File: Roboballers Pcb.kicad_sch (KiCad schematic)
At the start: 79 parts, among them U1 TSOP25xx, U1 Teensy4.1, U10 TSOP25xx, U11 TSOP25xx, U12 TSOP25xx, U13 MCP3008, U14 TSOP25xx, U15 TSOP25xx, U16 TSOP25xx, U17 TSOP25xx, U18 TSOP25xx, U19 TSOP25xx, U2 TSOP25xx, U20 TSOP25xx, U21 TSOP25xx, U22 MCP3008, U23 TSOP25xx, U24 TSOP25xx, U25 TSOP25xx, U26 TSOP25xx, U3 TSOP25xx, U4 TSOP25xx, U5 TSOP25xx, U6 MCP3008, U6 TSOP25xx, U7 TSOP25xx, U8 TSOP25xx, U9 TSOP25xx

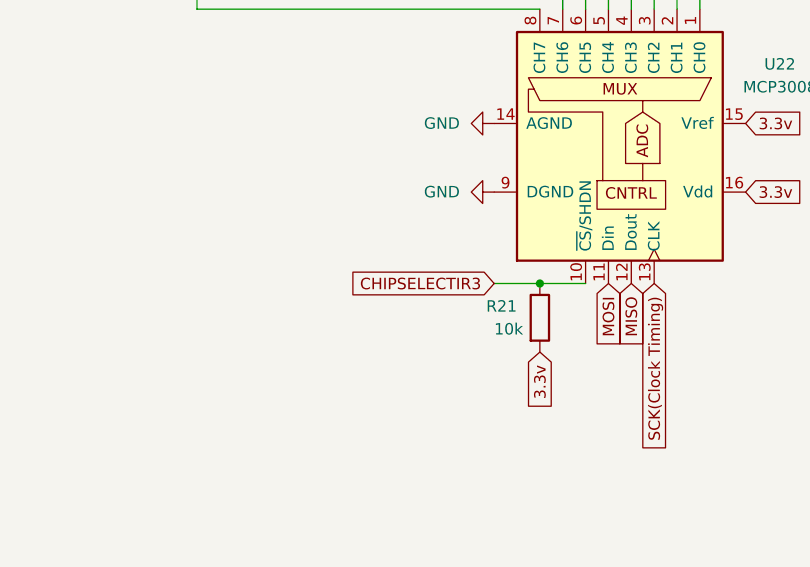
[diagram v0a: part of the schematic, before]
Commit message: Testing
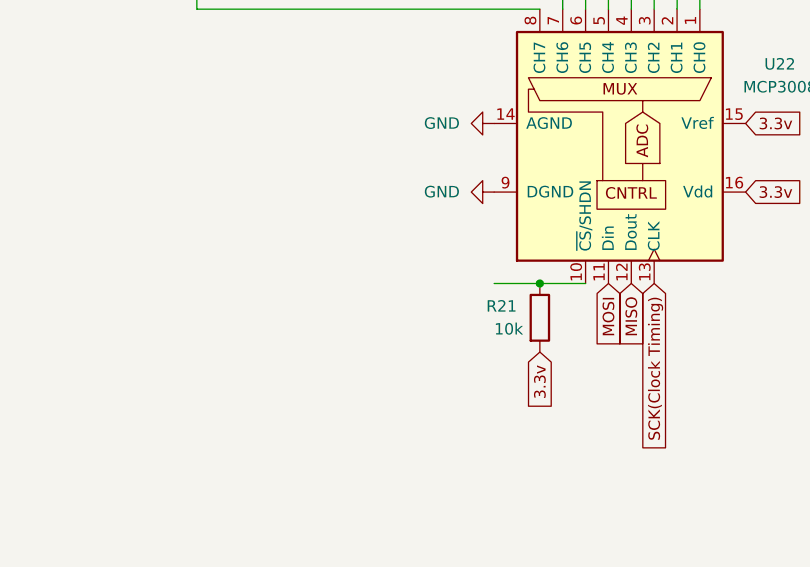
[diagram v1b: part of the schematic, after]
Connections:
- net CHIPSELECTIR3: no longer R21.1, U22.10 (~{CS}/SHDN)
- new net: R21.1, U22.10 (~{CS}/SHDN)
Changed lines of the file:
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@@
-		)
-	)
-	(global_label "CHIPSELECTIR3"
-		(shape input)
-		(at 302.26 146.05 180)
-		(fields_autoplaced yes)
-		(effects
-			(font
-				(size 1.27 1.27)
-			)
-			(justify right)
-		)
-		(property "Intersheetrefs" "${INTERSHEET_REFS}"
-			(at 284.942 146.05 0)
-			(effects
-				(font
-					(size 1.27 1.27)
-				)
-				(justify right)
-				(hide yes)
-			)
 		)
 	)

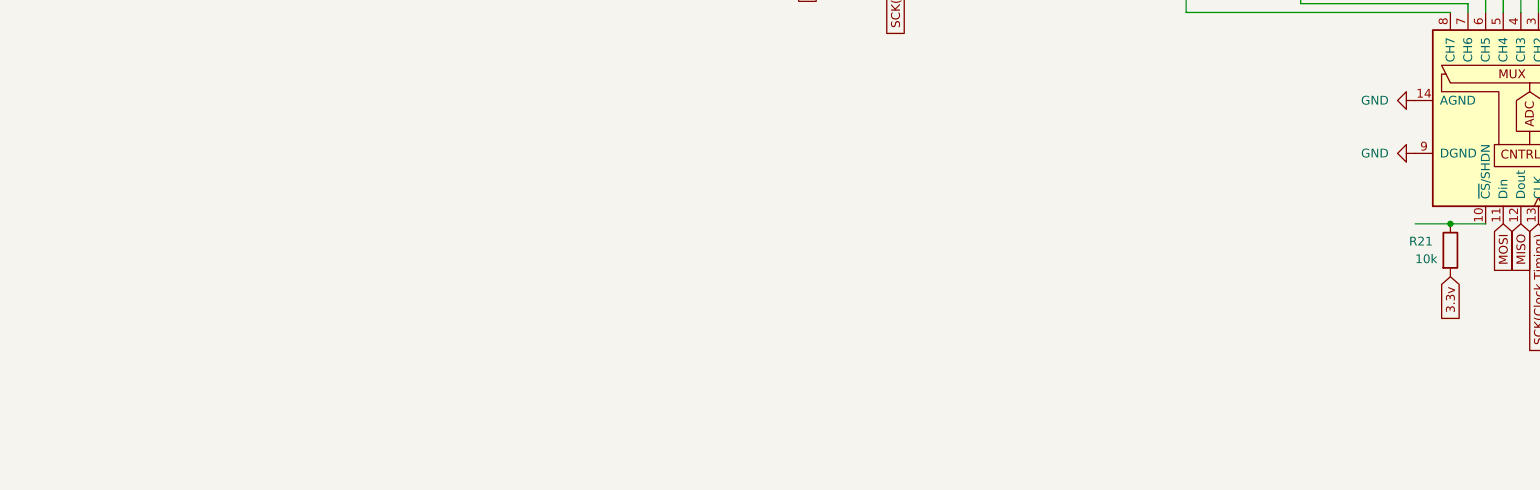
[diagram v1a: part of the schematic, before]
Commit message: Started on motor driver
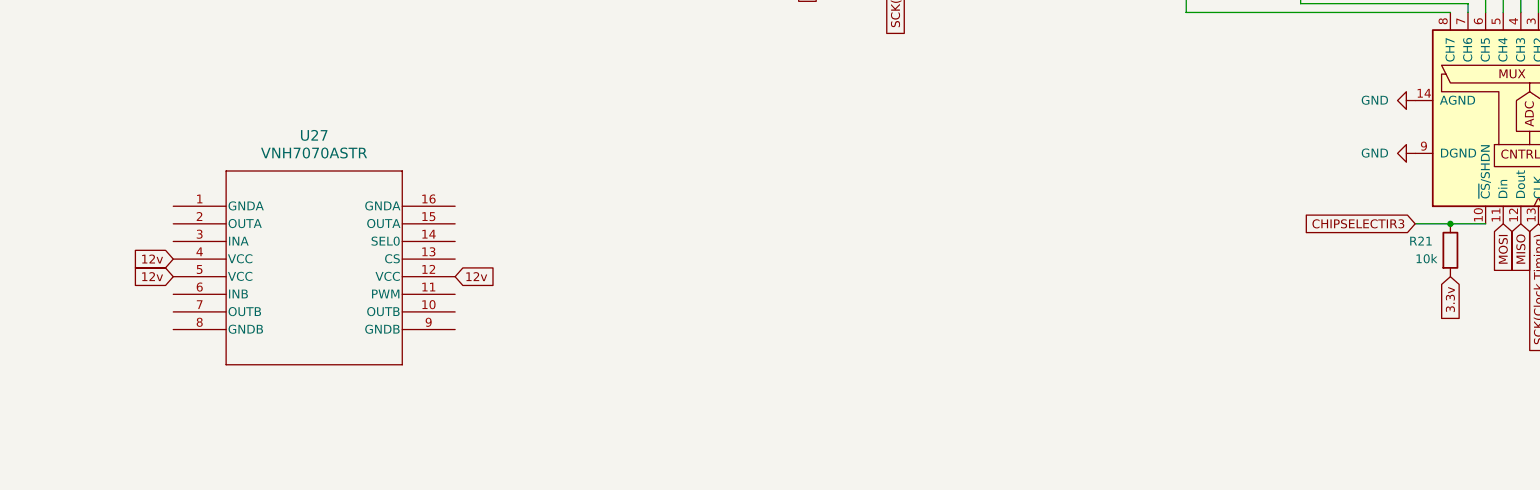
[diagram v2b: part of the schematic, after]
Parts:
- added U27: VNH7070ASTR, SO_0ASTR_STM, symbol Roboballers Symbol Libary:VNH7070ASTR
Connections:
- net CHIPSELECTIR3: now also R21.1, U22.10 (~{CS}/SHDN)
- new net 12v: U27.12 (VCC), U27.4 (VCC), U27.5 (VCC)
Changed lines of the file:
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@@
 		)
 	)
+	(global_label "12v"
+		(shape input)
+		(at 163.83 153.67 0)
+		(fields_autoplaced yes)
+		(effects
+			(font
+				(size 1.27 1.27)
+			)
+			(justify left)
+		)
+		(property "Intersheetrefs" "${INTERSHEET_REFS}"
+			(at 170.2018 153.67 0)
+			(effects
+				(font
+					(size 1.27 1.27)
+				)
+				(justify left)
+				(hide yes)
+			)
+		)
+	)
 	(global_label "3.3v"
 		(shape input)
@@
 		)
 	)
+	(global_label "12v"
+		(shape input)
+		(at 123.19 153.67 180)
+		(fields_autoplaced yes)
+		(effects
+			(font
+				(size 1.27 1.27)
+			)
+			(justify right)
+		)
+		(property "Intersheetrefs" "${INTERSHEET_REFS}"
+			(at 116.8182 153.67 0)
+			(effects
+				(font
+					(size 1.27 1.27)
+				)
+				(justify right)
+				(hide yes)
+			)
+		)
+	)
 	(global_label "3.3v"
 		(shape input)
@@
 		)
 	)
+	(global_label "12v"
+		(shape input)
+		(at 123.19 151.13 180)
+		(fields_autoplaced yes)
+		(effects
+			(font
+				(size 1.27 1.27)
+			)
+			(justify right)
+		)
+		(property "Intersheetrefs" "${INTERSHEET_REFS}"
+			(at 116.8182 151.13 0)
+			(effects
+				(font
+					(size 1.27 1.27)
+				)
+				(justify right)
+				(hide yes)
+			)
+		)
+	)
 	(global_label "3.3v"
 		(shape input)
@@
 		)
 	)
+	(global_label "CHIPSELECTIR3"
+		(shape input)
+		(at 302.26 146.05 180)
+		(fields_autoplaced yes)
+		(effects
+			(font
+				(size 1.27 1.27)
+			)
+			(justify right)
+		)
+		(property "Intersheetrefs" "${INTERSHEET_REFS}"
+			(at 284.942 146.05 0)
+			(effects
+				(font
+					(size 1.27 1.27)
+				)
+				(justify right)
+				(hide yes)
+			)
+		)
+	)
 	(global_label "3.3v"
 		(shape input)
@@
 					(unit 1)
 				)
+			)
+		)
+	)
+	(symbol
+		(lib_id "Roboballers Symbol Libary:VNH7070ASTR")
+		(at 123.19 143.51 0)
+		(unit 1)
+		(exclude_from_sim no)
+		(in_bom yes)
+		(on_board yes)
+		(dnp no)
+		(fields_autoplaced yes)
+		(property "Reference" "U27"
+			(at 143.51 133.35 0)
+			(effects
+				(font
+					(size 1.524 1.524)
+				)
+			)
+		)
+		(property "Value" "VNH7070ASTR"
+			(at 143.51 135.89 0)
+			(effects
+				(font
+					(size 1.524 1.524)
+				)
+			)
+		)
+		(property "Footprint" "SO_0ASTR_STM"
+			(at 163.576 140.208 0)
+			(effects
+				(font
+					(size 1.27 1.27)
+					(italic yes)
+				)
+				(hide yes)
+			)
+		)
+		(property "Datasheet" "VNH7070ASTR"
+			(at 123.444 139.954 0)
+			(effects
+				(font
+					(size 1.27 1.27)
+					(italic yes)
+				)
+				(hide yes)
+			)
+		)
+		(property "Description" ""
+			(at 123.19 143.51 0)
+			(effects
+				(font
+					(size 1.27 1.27)
+				)
+				(hide yes)
+			)
+		)
+		(pin "6"
+		)
+		(pin "1"
+		)
+		(pin "14"
+		)
+		(pin "16"
+		)
+		(pin "4"
+		)
+		(pin "2"
+		)
+		(pin "8"
+		)
+		(pin "12"
+		)
+		(pin "7"
+		)
+		(pin "11"
+		)
+		(pin "13"
+		)
+		(pin "10"
+		)
+		(pin "15"
+		)
+		(pin "5"
+		)
+		(pin "9"
+		)
+		(pin "3"
+		)
+		(instances
+			(project ""
+				(path "/0cb48458-5809-4c8b-a36b-a60cae24f4cb"
+					(reference "U27")
+					(unit 1)
+				)

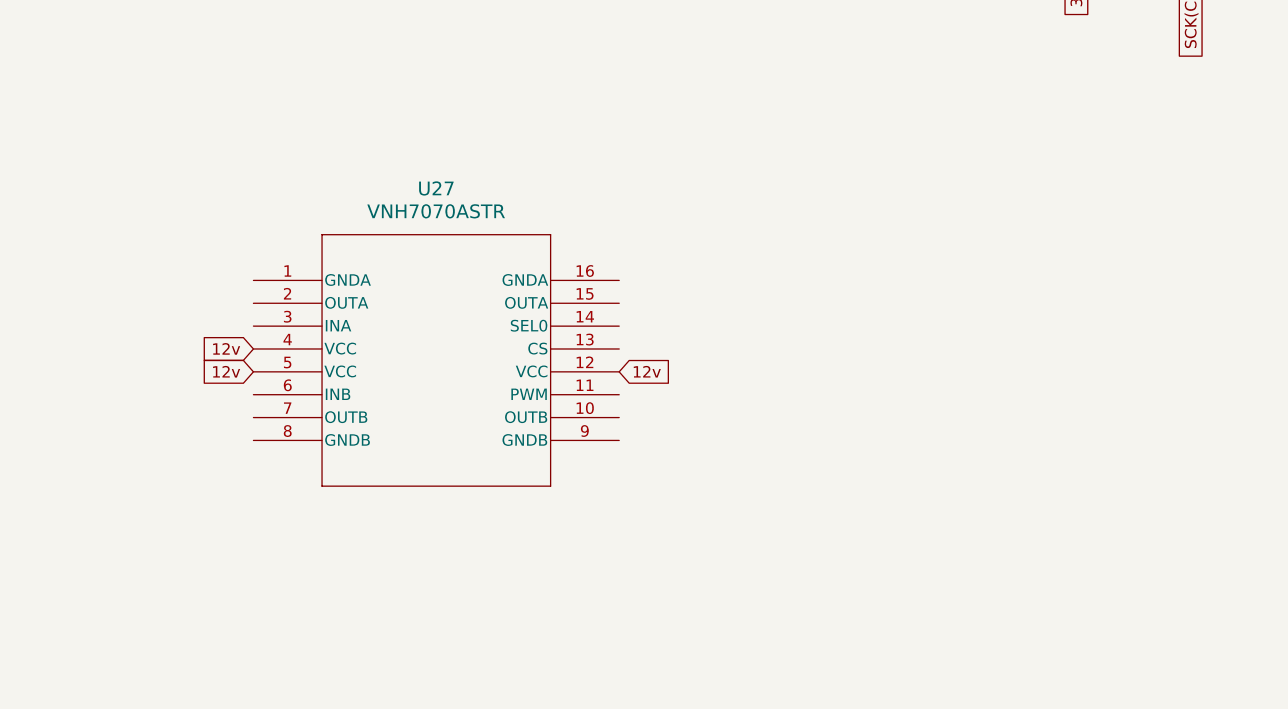
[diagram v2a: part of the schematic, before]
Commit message: PS - MotorDriver Work
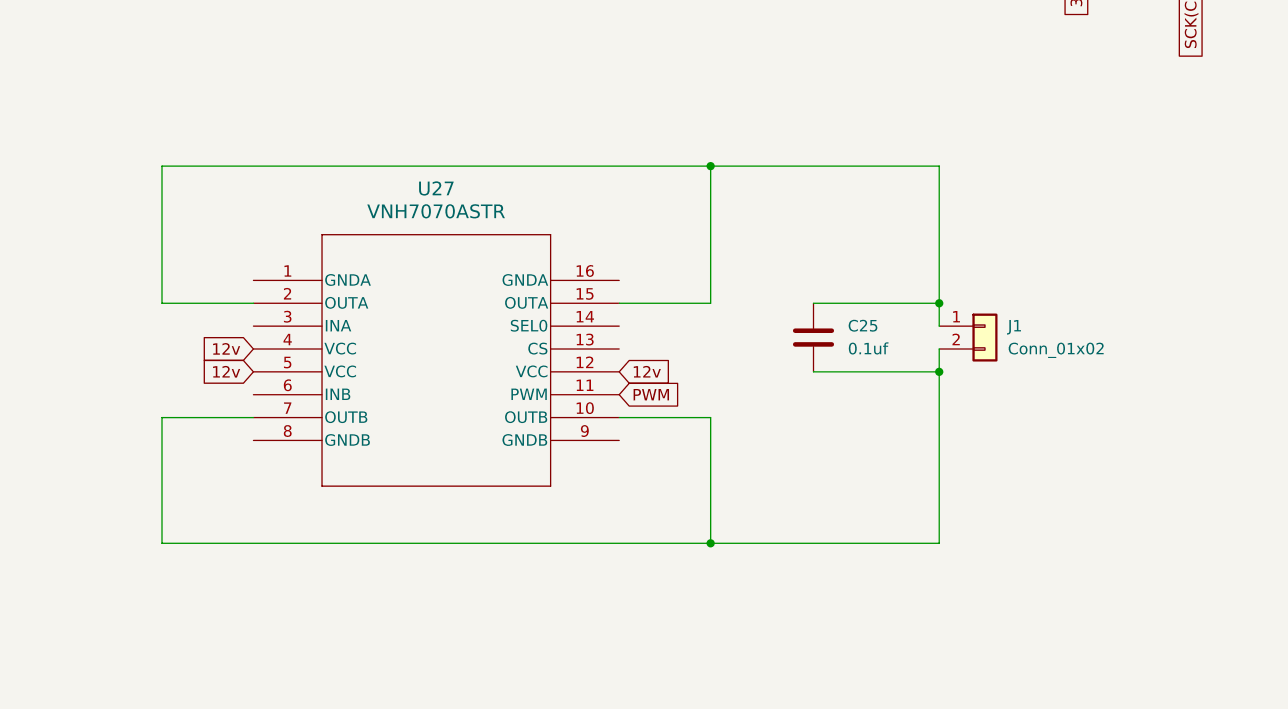
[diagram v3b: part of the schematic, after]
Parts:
- added C25: 0.1uf, Capacitor_SMD:C_0603_1608Metric, symbol Device:C
- added J1: Conn_01x02, symbol Connector_Generic:Conn_01x02
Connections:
- net at U27.10 (OUTB): now also U27.7 (OUTB), C25.2, J1.2 (Pin_2)
- net PWM: now reaches U27.11 (PWM)
- net at U27.15 (OUTA): now also U27.2 (OUTA), C25.1, J1.1 (Pin_1)

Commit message: Full pcb
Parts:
- removed R0: 10k, Resistor_THT:R_Axial_DIN0207_L6.3mm_D2.5mm_P10.16mm_Horizontal, symbol Device:R
- removed U1: Teensy4.1, symbol teensy:Teensy4.1
- removed U1, U11, U12, U15, U17, U2, U3, U4, U5, U7: TSOP25xx, PSR IR Sensors:TSSP4038, symbol Interface_Optical:TSOP25xx
- removed U13, U22, U6: MCP3008, Package_DIP:DIP-16_W7.62mm, symbol Analog_ADC:MCP3008
- removed U27: VNH7070ASTR, SO_0ASTR_STM, symbol Roboballers Symbol Libary:VNH7070ASTR
- added C26, C27, C28: 0.1uf, Capacitor_SMD:C_0603_1608Metric, symbol Device:C
- added J2, J3, J4: Conn_01x02, symbol Connector_Generic:Conn_01x02
- added J5: Screw_Terminal_01x02, TerminalBlock_Phoenix:TerminalBlock_Phoenix_PT-1,5-2-5.0-H_1x02_P5.00mm_Horizontal, symbol Connector:Screw_Terminal_01x02
- added J6: Conn_01x02, PSR-Headers:1x02-Header, symbol Connector_Generic:Conn_01x02
- added R27, R29, R31, R32, R33, R34, R35, R36, R37, R38, R39: 100k, PSR Resistors:R_0805_2012Metric_100k, symbol Device:R
- added R28, R30: 10k, Resistor_THT:R_Axial_DIN0207_L6.3mm_D2.5mm_P10.16mm_Horizontal, symbol Device:R
- added U1, U2, U3, U4: VNH7070ASTR, SO_0ASTR_STM, symbol 2024-10-18_00-41-23:VNH7070ASTR
- added U11: OpenMV_H7_R2, OpenMV:OpenMV, symbol OpenMV:OpenMV_H7_R2
- added U12, U27, U28: MCP3008, Package_DIP:DIP-16_W7.62mm, symbol Analog_ADC:MCP3008
- added U13, U22, U29, U30, U31, U32, U33, U34, U35, U36: TSOP25xx, PSR IR Sensors:TSSP4038, symbol Interface_Optical:TSOP25xx
- added U15: SEN0140, CompassSensor:LIS3MDL, symbol Compass_Sensor:SEN0140
- added U17: RockerSwitch, RockerSwitch:RockerSwitch-PSR, symbol RockerSwitch:RockerSwitch
- added U5: Teensy4.1, symbol teensy:Teensy4.1
- added U7: V_Regulator_-_5v, TerminalBlock_Phoenix:TerminalBlock_Phoenix_PT-1,5-4-5.0-H_1x04_P5.00mm_Horizontal, symbol Voltage Regulator:V_Regulator_-_5v
- C1, C2, C3, C4: footprint Capacitor_SMD:C_0603_1608Metric -> (none)
- R1, R10, R11, R2, R3, R4, R5, R6, R7, R8, R9: value 100k -> 100; footprint PSR Resistors:R_0805_2012Metric_100k -> (none)
- R12: value 10k -> 100; footprint Resistor_THT:R_Axial_DIN0207_L6.3mm_D2.5mm_P10.16mm_Horizontal -> (none)
- R16: value 100k -> 10k; footprint PSR Resistors:R_0805_2012Metric_100k -> Resistor_THT:R_Axial_DIN0207_L6.3mm_D2.5mm_P10.16mm_Horizontal
- R21: value 10k -> 100k; footprint Resistor_THT:R_Axial_DIN0207_L6.3mm_D2.5mm_P10.16mm_Horizontal -> PSR Resistors:R_0805_2012Metric_100k
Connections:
- net 12v: now also U1.12 (VCC), U1.4 (VCC), U1.5 (VCC), U17.2 (ACC), U2.12 (VCC), U2.4 (VCC), U2.5 (VCC), U3.12 (VCC), U3.4 (VCC), U3.5 (VCC), U4.12 (VCC), U4.4 (VCC), U4.5 (VCC), U7.1 (IN+)
- net 3.3v: now also R16.2, R28.2, R30.2, U12.15 (Vref), U12.16 (Vdd), U13.3 (GND), U15.1 (3.3v), U22.3 (GND), U27.15 (Vref), U27.16 (Vdd), U28.15 (Vref), U28.16 (Vdd), U29.3 (GND), U30.3 (GND), U31.3 (GND), U32.3 (GND), U33.3 (GND), U34.3 (GND), U35.3 (GND), U36.3 (GND), U5.46 (3V3); no longer R12.2, R21.2
- net CHIPSELECTIR1: now also R16.1, U12.10 (~{CS}/SHDN), U5.30 (38_CS1_IN1)
- net CHIPSELECTIR2: now also R30.1, U28.10 (~{CS}/SHDN), U5.29 (37_CS); no longer R12.1
- net CHIPSELECTIR3: now also U5.28 (36_CS); no longer R21.1
- net GND: now also C25.2, U24.2 (Vs), U25.2 (Vs), U26.2 (Vs), U6.2 (Vs), U8.2 (Vs), C26.2, C27.2, C28.2, J5.1 (Pin_1), J6.2 (Pin_2), U1.1 (GNDA), U1.16 (GNDA), U1.8 (GNDB), U1.9 (GNDB), U11.9 (GND), U12.14 (AGND), U12.9 (DGND), U13.2 (Vs), U15.2 (GND), U17.3 (GND), U2.1 (GNDA), U2.16 (GNDA), U2.8 (GNDB), U2.9 (GNDB), U22.2 (Vs), U27.14 (AGND), U27.9 (DGND), U28.14 (AGND), U28.9 (DGND), U29.2 (Vs), U3.1 (GNDA), U3.16 (GNDA), U3.8 (GNDB), U3.9 (GNDB), U30.2 (Vs), U4.1 (GNDA), U4.16 (GNDA), U4.8 (GNDB), U4.9 (GNDB), U5.1 (GND), U5.47 (GND), U7.2 (IN-), U7.4 (OUT-); no longer C1.2, C2.2, C3.2, C4.2, U14.2 (Vs), U18.2 (Vs)
- net MISO: now also U12.12 (Dout), U27.12 (Dout), U28.12 (Dout), U5.14 (12_MISO_MQSL)
- net MOSI: now also U12.11 (Din), U27.11 (Din), U28.11 (Din), U5.13 (11_MOSI_CTX1)
- net SCK(Clock Timing): now also U12.13 (CLK), U27.13 (CLK), U28.13 (CLK), U5.35 (13_SCK_LED)
- net at U21.1 (OUT): now also R24.1; no longer R22.1
- net at R22.2: now also C13.1, U27.8 (CH7); no longer C20.1
- net at C21.1: now also R32.2, U27.4 (CH3); no longer R23.2
- net at R26.1: now also U23.1 (OUT); no longer U26.1 (OUT)
- net at R23.1: now also U20.1 (OUT); no longer U23.1 (OUT)
- net Direction2(1): now reaches R2.1
- net Direction2(1): now also U5.5 (3_LRCLK2)
- net at R18.1: now also U13.1 (OUT); no longer U18.1 (OUT)
- net at R11.1: now also U3.11 (PWM)
- net at R15.1: now also U9.1 (OUT)
- net at R8.2: now also U4.6 (INB); no longer C8.1
- net at R7.2: now also U4.3 (INA); no longer C7.1
- net at C6.1: now also R14.2, U12.7 (CH6); no longer R6.2
- net at C5.1: now also R13.2, U12.8 (CH7); no longer R5.2
- net at C4.1: now also J4.1 (Pin_1), U4.15 (OUTA), U4.2 (OUTA); no longer R4.2
- net at C3.1: now also J3.1 (Pin_1), U3.15 (OUTA), U3.2 (OUTA); no longer R3.2
- net at R2.2: now also U1.6 (INB); no longer C2.1
- net at C1.1: now also J1.1 (Pin_1), U1.15 (OUTA), U1.2 (OUTA); no longer R1.2
- net at R17.1: now also U10.1 (OUT)
- net at C11.1: now also R20.2, U12.2 (CH1); no longer R11.2
- net Direction1(4): now reaches R7.1
- net Direction1(4): now also U5.23 (31_CTX3)
- net at R26.2: now also C17.1, U27.6 (CH5); no longer C24.1
- net at C23.1: now also R34.2, U27.3 (CH2); no longer R25.2
- net at R24.2: now also C15.1, U27.7 (CH6); no longer C22.1
- net at C19.1: now also R29.2, U27.5 (CH4); no longer R20.2
- net at R19.2: now also C10.1, U12.3 (CH2); no longer C18.1
- net at R18.2: now also C9.1, U12.4 (CH3); no longer C17.1
- net at R10.1: now also U2.11 (PWM); no longer U10.1 (OUT)
- net PWM1: now reaches R9.2
- net PWM1: now also U5.42 (20_A6_TX5_LRCLK1); no longer C9.1
- net at R20.1: now also U16.1 (OUT); no longer U20.1 (OUT)
- net at R9.1: now also U1.11 (PWM); no longer U9.1 (OUT)
- net at R15.2: now also C7.1, U12.6 (CH5); no longer C14.1
- net at U8.1 (OUT): now also R14.1; no longer R8.1
- net at C12.1: now also R21.2, U12.1 (CH0); no longer R13.2
- net Direction1(3): now reaches R3.1
- net Direction1(3): now also U5.8 (6_OUT1D)
- net PWM3: now reaches R10.2
- net PWM3: now also U5.44 (22_A8_CTX1); no longer C10.1
- net at U6.1 (OUT): now also R13.1; no longer R6.1
- net at C25.1: now also R36.2, U27.2 (CH1); no longer J1.1 (Pin_1)
- net at J1.2 (Pin_2): now also C1.2, U1.10 (OUTB), U1.7 (OUTB); no longer C25.2
- net at U14.1 (OUT): now also R19.1; no longer R14.1
- net Direction2(3): now reaches R4.1
- net Direction2(3): now also U5.11 (9_OUT1C)
- net at U24.1 (OUT): now also R27.1; no longer R24.1
- net at U25.1 (OUT): now also R29.1; no longer R25.1
- net Direction1(1): now reaches R1.1
- net Direction1(1): now also U5.4 (2_OUT2)
- net at U19.1 (OUT): now also R22.1; no longer R19.1
- net Direction1(2): now reaches R5.1
- net Direction1(2): now also U5.6 (4_BCLK2)
- net at R17.2: now also C8.1, U12.5 (CH4); no longer C16.1
- new net: R36.1, U33.1 (OUT)
- new net: R39.1, U36.1 (OUT)
- new net: C4.2, J4.2 (Pin_2), U4.10 (OUTB), U4.7 (OUTB)
- new net: R12.1, U4.11 (PWM)
- new net: C3.2, J3.2 (Pin_2), U3.10 (OUTB), U3.7 (OUTB)
- new net: R33.1, U30.1 (OUT)
- new net: C27.1, R38.2, U27.1 (CH0)
- new net: R28.1, U27.10 (~{CS}/SHDN)
- new net: C14.1, R23.2, U28.8 (CH7)
- new net: J5.2 (Pin_2), J6.1 (Pin_1), U17.1 (Power)
- new net: R37.1, U34.1 (OUT)
- new net: R34.1, U31.1 (OUT)
- new net: R31.1, U26.1 (OUT)
- new net: C18.1, R27.2, U28.6 (CH5)
- new net: R25.1, U22.1 (OUT)
- new net: R5.2, U3.3 (INA)
- new net: R6.2, U3.6 (INB)
- new net: C28.1, R39.2, U28.1 (CH0)
- new net: C22.1, R33.2, U28.4 (CH3)
- new net: C16.1, R25.2, U28.7 (CH6)
- new net: R35.1, U32.1 (OUT)
- new net: R1.2, U1.3 (INA)
- new net: C20.1, R31.2, U28.5 (CH4)
- new net: R38.1, U35.1 (OUT)
- new net: C26.1, R37.2, U28.2 (CH1)
- new net: C24.1, R35.2, U28.3 (CH2)
- new net: C2.2, J2.2 (Pin_2), U2.10 (OUTB), U2.7 (OUTB)
- new net: C2.1, J2.1 (Pin_1), U2.15 (OUTA), U2.2 (OUTA)
- new net: R3.2, U2.3 (INA)
- new net: R4.2, U2.6 (INB)
- new net: R32.1, U29.1 (OUT)
- new net: R21.1, U18.1 (OUT)
- new net 5v: U11.10 (VIN), U5.48 (VIN), U7.3 (OUT+)
- new net Direction2(2): R6.1, U5.7 (5_IN2)
- new net Direction2(4): R8.1, U5.24 (32_OUT1B)
- new net PWM2: R11.2, U5.43 (21_A7_RX5_BCLK1)
- new net PWM4: R12.2, U5.45 (23_A9_CRX1_MCLK1)
- new net RX: U11.2 (P2), U5.2 (0_RX1_CRX2_CS1)
- new net SCL: U15.3 (SCL), U5.41 (19_A5_SCL)
- new net SDA: U15.4 (SDA), U5.40 (18_A4_SDA)
- new net TX: U11.1 (P1), U5.3 (1_TX1_CTX2_MISO1)
- no-connect marks 0 -> 8
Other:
- note added: "Voltmeter"

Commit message: Added some Footprints
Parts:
- C1, C2, C3, C4: footprint (none) -> Capacitor_SMD:C_0603_1608Metric
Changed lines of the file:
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@@
 			)
 		)
-		(property "Footprint" ""
+		(property "Footprint" "Capacitor_SMD:C_0603_1608Metric"
 			(at 102.5652 118.11 0)
 			(effects
@@
 			)
 		)
-		(property "Footprint" ""
+		(property "Footprint" "Capacitor_SMD:C_0603_1608Metric"
 			(at 103.8352 35.56 0)
 			(effects
@@
 			)
 		)
-		(property "Footprint" ""
+		(property "Footprint" "Capacitor_SMD:C_0603_1608Metric"
 			(at 102.5652 77.47 0)
 			(effects
@@
 			)
 		)
-		(property "Footprint" ""
+		(property "Footprint" "Capacitor_SMD:C_0603_1608Metric"
 			(at 101.2952 157.48 0)
 			(effects
